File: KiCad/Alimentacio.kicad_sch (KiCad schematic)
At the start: 6 parts

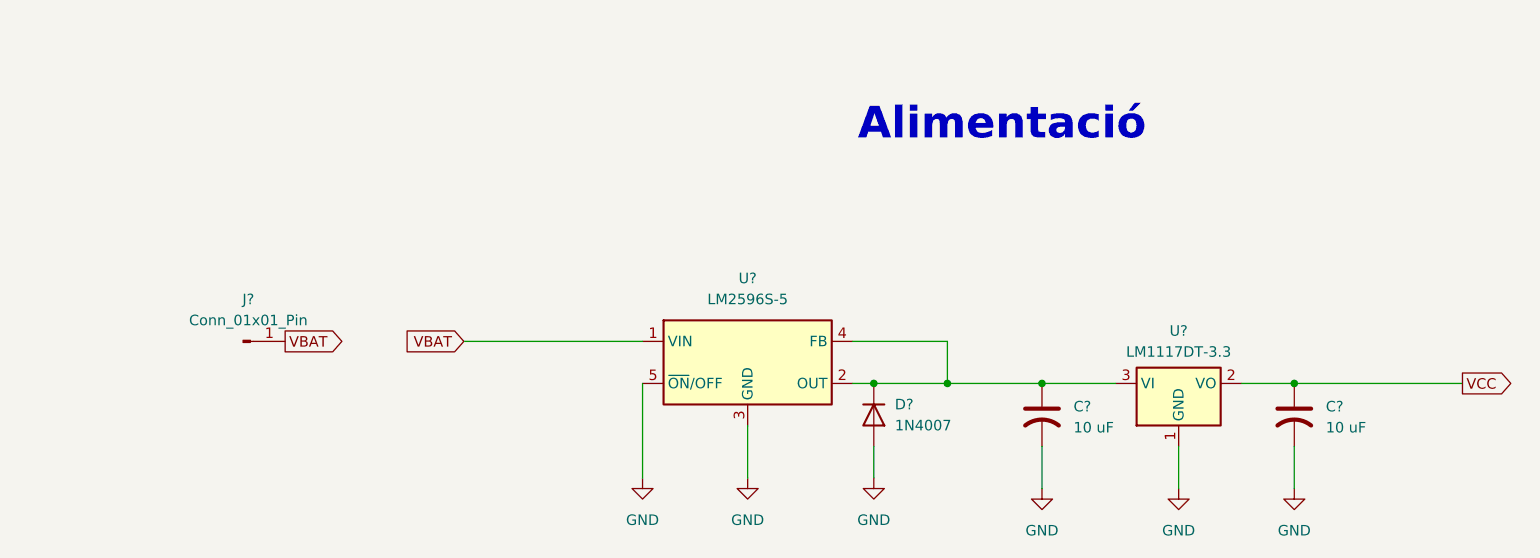
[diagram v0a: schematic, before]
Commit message: Solucionando problemas del esquematic
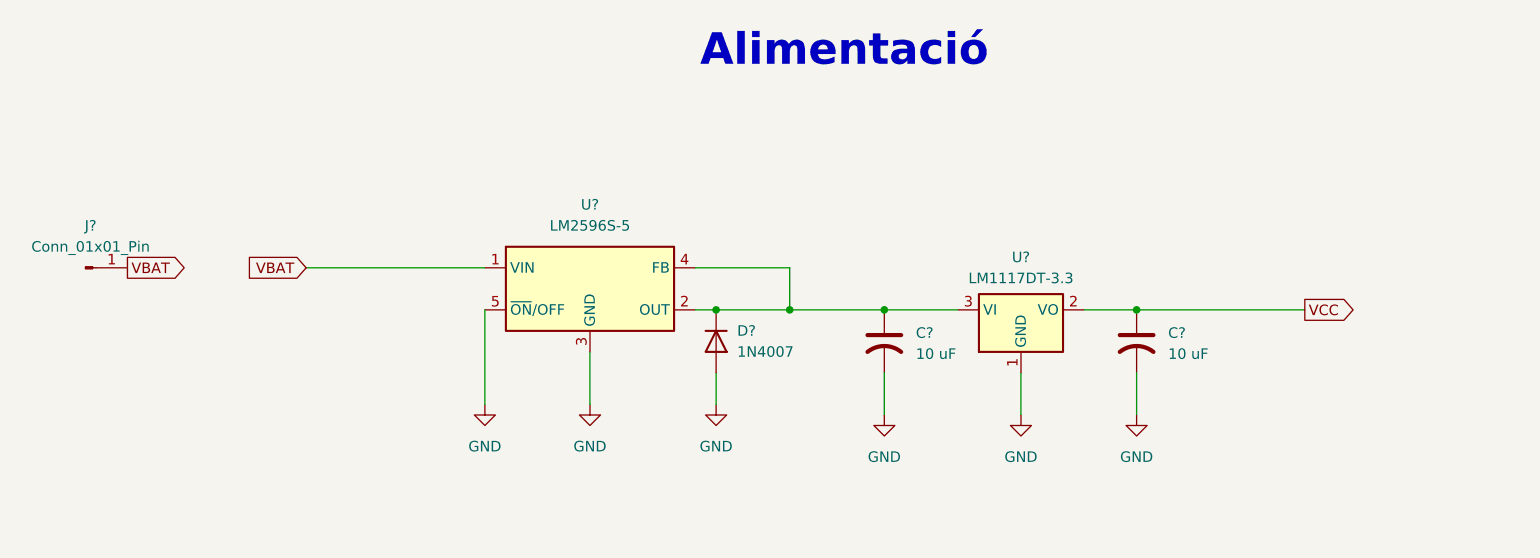
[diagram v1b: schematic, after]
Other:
- title: edd-project-grup-dimecres-dc_d_llums -> Alimentacio
- moved on the sheet: C?, D?, J?, U?

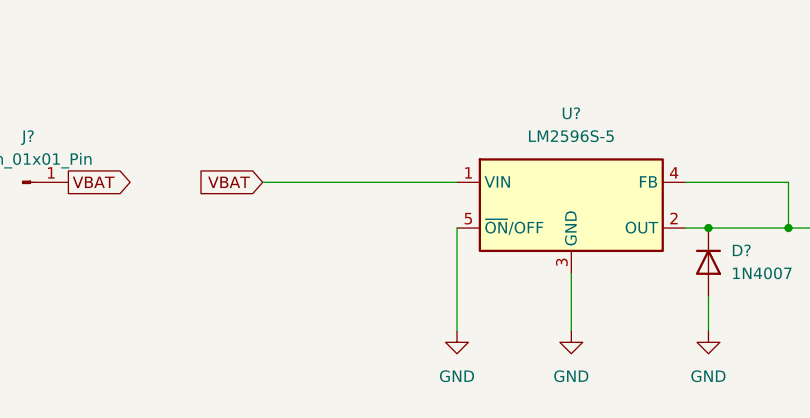
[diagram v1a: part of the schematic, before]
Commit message: Capacitat DC/DC
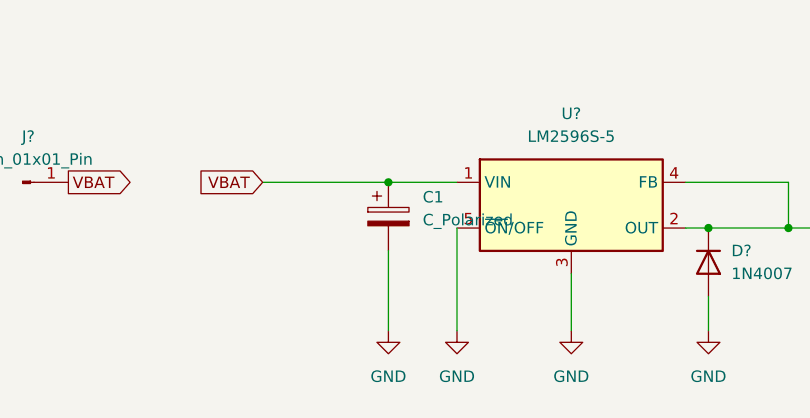
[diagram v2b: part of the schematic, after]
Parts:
- added C1: C_Polarized, symbol Device:C_Polarized
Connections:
- net GND: now also C1.2
- net VBAT: now also C1.1
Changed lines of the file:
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@@
+	)
+	(junction
+		(at 60.96 40.64)
+		(diameter 0)
+		(color 0 0 0 0)
 	)
 	(junction
@@
 	(wire
 		(pts
+			(xy 60.96 48.26) (xy 60.96 57.15)
+		)
+		(stroke
+			(width 0)
+			(type default)
+		)
+	)
+	(wire
+		(pts
 			(xy 140.97 45.72) (xy 147.32 45.72)
 		)
@@
 	(wire
 		(pts
-			(xy 46.99 40.64) (xy 68.58 40.64)
+			(xy 60.96 40.64) (xy 68.58 40.64)
+		)
+		(stroke
+			(width 0)
+			(type default)
+		)
+	)
+	(wire
+		(pts
+			(xy 46.99 40.64) (xy 60.96 40.64)
 		)
 		(stroke
@@
 		)
 		(instances
+			(project "Alimentacio"
+				(path "/6b132bbb-272b-40ab-bbcf-3d5da3f07086"
+					(reference "#PWR?")
+					(unit 1)
+				)
+			)
 			(project "Grup_D_Llums"
 				(path "/88ef36bc-9439-47f2-adb5-e1da6bb8c9dd/c965bb79-4e48-4b35-b9c7-2e902c1fe9a5"
@@
 		)
 		(instances
+			(project "Alimentacio"
+				(path "/6b132bbb-272b-40ab-bbcf-3d5da3f07086"
+					(reference "U?")
+					(unit 1)
+				)
+			)
 			(project "Grup_D_Llums"
 				(path "/88ef36bc-9439-47f2-adb5-e1da6bb8c9dd/c965bb79-4e48-4b35-b9c7-2e902c1fe9a5"
@@
 		)
 		(instances
+			(project "Alimentacio"
+				(path "/6b132bbb-272b-40ab-bbcf-3d5da3f07086"
+					(reference "#PWR?")
+					(unit 1)
+				)
+			)
 			(project "Grup_D_Llums"
 				(path "/88ef36bc-9439-47f2-adb5-e1da6bb8c9dd/c965bb79-4e48-4b35-b9c7-2e902c1fe9a5"
@@
 		)
 		(instances
+			(project "Alimentacio"
+				(path "/6b132bbb-272b-40ab-bbcf-3d5da3f07086"
+					(reference "U?")
+					(unit 1)
+				)
+			)
 			(project "Grup_D_Llums"
 				(path "/88ef36bc-9439-47f2-adb5-e1da6bb8c9dd/c965bb79-4e48-4b35-b9c7-2e902c1fe9a5"
@@
 	)
 	(symbol
+		(lib_id "power:GND")
+		(at 60.96 57.15 0)
+		(unit 1)
+		(exclude_from_sim no)
+		(in_bom yes)
+		(on_board yes)
+		(dnp no)
+		(fields_autoplaced yes)
+		(property "Reference" "#PWR01"
+			(at 60.96 63.5 0)
+			(effects
+				(font
+					(size 1.27 1.27)
+				)
+				(hide yes)
+			)
+		)
+		(property "Value" "GND"
+			(at 60.96 62.23 0)
+			(effects
+				(font
+					(size 1.27 1.27)
+				)
+			)
+		)
+		(property "Footprint" ""
+			(at 60.96 57.15 0)
+			(effects
+				(font
+					(size 1.27 1.27)
+				)
+				(hide yes)
+			)
+		)
+		(property "Datasheet" ""
+			(at 60.96 57.15 0)
+			(effects
+				(font
+					(size 1.27 1.27)
+				)
+				(hide yes)
+			)
+		)
+		(property "Description" "Power symbol creates a global label with name \"GND\" , ground"
+			(at 60.96 57.15 0)
+			(effects
+				(font
+					(size 1.27 1.27)
+				)
+				(hide yes)
+			)
+		)
+		(pin "1"
+		)
+		(instances
+			(project "Alimentacio"
+				(path "/6b132bbb-272b-40ab-bbcf-3d5da3f07086"
+					(reference "#PWR01")
+					(unit 1)
+				)
+			)
+		)
+	)
+	(symbol
 		(lib_id "Device:C_US")
 		(at 147.32 49.53 0)
@@
 		)
 		(instances
+			(project "Alimentacio"
+				(path "/6b132bbb-272b-40ab-bbcf-3d5da3f07086"
+					(reference "C?")
+					(unit 1)
+				)
+			)
 			(project "Grup_D_Llums"
 				(path "/88ef36bc-9439-47f2-adb5-e1da6bb8c9dd/c965bb79-4e48-4b35-b9c7-2e902c1fe9a5"
@@
 		)
 		(instances
+			(project "Alimentacio"
+				(path "/6b132bbb-272b-40ab-bbcf-3d5da3f07086"
+					(reference "#PWR?")
+					(unit 1)
+				)
+			)
 			(project "Grup_D_Llums"
 				(path "/88ef36bc-9439-47f2-adb5-e1da6bb8c9dd/c965bb79-4e48-4b35-b9c7-2e902c1fe9a5"
@@
 		)
 		(instances
+			(project "Alimentacio"
+				(path "/6b132bbb-272b-40ab-bbcf-3d5da3f07086"
+					(reference "J?")
+					(unit 1)
+				)
+			)
 			(project "Grup_D_Llums"
 				(path "/88ef36bc-9439-47f2-adb5-e1da6bb8c9dd/c965bb79-4e48-4b35-b9c7-2e902c1fe9a5"
@@
 		)
 		(instances
+			(project "Alimentacio"
+				(path "/6b132bbb-272b-40ab-bbcf-3d5da3f07086"
+					(reference "#PWR?")
+					(unit 1)
+				)
+			)
 			(project "Grup_D_Llums"
 				(path "/88ef36bc-9439-47f2-adb5-e1da6bb8c9dd/c965bb79-4e48-4b35-b9c7-2e902c1fe9a5"
@@
 		)
 		(instances
+			(project "Alimentacio"
+				(path "/6b132bbb-272b-40ab-bbcf-3d5da3f07086"
+					(reference "#PWR?")
+					(unit 1)
+				)
+			)
 			(project "Grup_D_Llums"
 				(path "/88ef36bc-9439-47f2-adb5-e1da6bb8c9dd/c965bb79-4e48-4b35-b9c7-2e902c1fe9a5"
@@
 		)
 		(instances
+			(project "Alimentacio"
+				(path "/6b132bbb-272b-40ab-bbcf-3d5da3f07086"
+					(reference "#PWR?")
+					(unit 1)
+				)
+			)
 			(project "Grup_D_Llums"
 				(path "/88ef36bc-9439-47f2-adb5-e1da6bb8c9dd/c965bb79-4e48-4b35-b9c7-2e902c1fe9a5"
@@
 		)
 		(instances
+			(project "Alimentacio"
+				(path "/6b132bbb-272b-40ab-bbcf-3d5da3f07086"
+					(reference "D?")
+					(unit 1)
+				)
+			)
 			(project "Grup_D_Llums"
 				(path "/88ef36bc-9439-47f2-adb5-e1da6bb8c9dd/c965bb79-4e48-4b35-b9c7-2e902c1fe9a5"
@@
 	)
 	(symbol
+		(lib_id "Device:C_Polarized")
+		(at 60.96 44.45 0)
+		(unit 1)
+		(exclude_from_sim no)
+		(in_bom yes)
+		(on_board yes)
+		(dnp no)
+		(fields_autoplaced yes)
+		(property "Reference" "C1"
+			(at 64.77 42.2909 0)
+			(effects
+				(font
+					(size 1.27 1.27)
+				)
+				(justify left)
+			)
+		)
+		(property "Value" "C_Polarized"
+			(at 64.77 44.8309 0)
+			(effects
+				(font
+					(size 1.27 1.27)
+				)
+				(justify left)
+			)
+		)
+		(property "Footprint" ""
+			(at 61.9252 48.26 0)
+			(effects
+				(font
+					(size 1.27 1.27)
+				)
+				(hide yes)
+			)
+		)
+		(property "Datasheet" "~"
+			(at 60.96 44.45 0)
+			(effects
+				(font
+					(size 1.27 1.27)
+				)
+				(hide yes)
+			)
+		)
+		(property "Description" "Polarized capacitor"
+			(at 60.96 44.45 0)
+			(effects
+				(font
+					(size 1.27 1.27)
+				)
+				(hide yes)
+			)
+		)
+		(pin "2"
+		)
+		(pin "1"
+		)
+		(instances
+			(project ""
+				(path "/6b132bbb-272b-40ab-bbcf-3d5da3f07086"
+					(reference "C1")
+					(unit 1)
+				)
+			)
+		)
+	)
+	(symbol
 		(lib_id "Device:C_US")
 		(at 116.84 49.53 0)
@@
 		)
 		(instances
+			(project "Alimentacio"
+				(path "/6b132bbb-272b-40ab-bbcf-3d5da3f07086"
+					(reference "C?")
+					(unit 1)
+				)
+			)
 			(project "Grup_D_Llums"
 				(path "/88ef36bc-9439-47f2-adb5-e1da6bb8c9dd/c965bb79-4e48-4b35-b9c7-2e902c1fe9a5"
@@
 		)
 	)
+	(sheet_instances
+		(path "/"
+			(page "1")
+		)
+	)
+	(embedded_fonts no)
 )
